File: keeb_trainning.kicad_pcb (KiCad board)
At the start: 2 copper layers, 0 parts

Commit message: :construction: WIP: Redraw wires
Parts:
- added D1: Diode, ScottoKeebs_Components:Diode_SOD-123, F.Cu at (72.5, 81.9)
- added D10: Diode, ScottoKeebs_Components:Diode_SOD-123, F.Cu at (59.1, 87.7)
- added D11: Diode, ScottoKeebs_Components:Diode_SOD-123, F.Cu at (72.5, 93.4)
- added D12: Diode, ScottoKeebs_Components:Diode_SOD-123, F.Cu at (69.2, 93.4)
- added D13: Diode, ScottoKeebs_Components:Diode_SOD-123, F.Cu at (65.8, 93.4)
- added D14: Diode, ScottoKeebs_Components:Diode_SOD-123, F.Cu at (62.5, 93.4)
- added D15: Diode, ScottoKeebs_Components:Diode_SOD-123, F.Cu at (59.1, 93.4)
- added D16: Diode, ScottoKeebs_Components:Diode_SOD-123, F.Cu at (72.5, 99.2)
- added D17: Diode, ScottoKeebs_Components:Diode_SOD-123, F.Cu at (69.2, 99.2)
- added D18: Diode, ScottoKeebs_Components:Diode_SOD-123, F.Cu at (65.8, 99.2)
- added D19: Diode, ScottoKeebs_Components:Diode_SOD-123, F.Cu at (62.5, 99.2)
- added D2: Diode, ScottoKeebs_Components:Diode_SOD-123, F.Cu at (69.2, 81.9)
- added D20: Diode, ScottoKeebs_Components:Diode_SOD-123, F.Cu at (59.1, 99.2)
- added D3: Diode, ScottoKeebs_Components:Diode_SOD-123, F.Cu at (65.8, 81.9)
- added D4: Diode, ScottoKeebs_Components:Diode_SOD-123, F.Cu at (62.5, 81.9)
- added D5: Diode, ScottoKeebs_Components:Diode_SOD-123, F.Cu at (59.1, 81.9)
- added D6: Diode, ScottoKeebs_Components:Diode_SOD-123, F.Cu at (72.5, 87.7)
- added D7: Diode, ScottoKeebs_Components:Diode_SOD-123, F.Cu at (69.2, 87.7)
- added D8: Diode, ScottoKeebs_Components:Diode_SOD-123, F.Cu at (65.8, 87.7)
- added D9: Diode, ScottoKeebs_Components:Diode_SOD-123, F.Cu at (62.5, 87.7)
- added S1: Keyswitch, ScottoKeebs_Choc:Choc_V2, F.Cu at (88.2, 53.7)
- added S10: Keyswitch, ScottoKeebs_Choc:Choc_V2, F.Cu at (145.7, 69.7)
- added S11: Keyswitch, ScottoKeebs_Choc:Choc_V2, F.Cu at (166.2, 74.2)
- added S12: Keyswitch, ScottoKeebs_Choc:Choc_V2, F.Cu at (185.2, 75.8)
- added S13: Keyswitch, ScottoKeebs_Choc:Choc_V2, F.Cu at (87.7, 89.7)
- added S14: Keyswitch, ScottoKeebs_Choc:Choc_V2, F.Cu at (106.7, 89.8)
- added S15: Keyswitch, ScottoKeebs_Choc:Choc_V2, F.Cu at (126.2, 83.8)
- added S16: Keyswitch, ScottoKeebs_Choc:Choc_V2, F.Cu at (145.7, 87.8)
- added S17: Keyswitch, ScottoKeebs_Choc:Choc_V2, F.Cu at (166.2, 92.3)
- added S18: Keyswitch, ScottoKeebs_Choc:Choc_V2, F.Cu at (185.2, 94.3)
- added S19: Keyswitch, ScottoKeebs_Choc:Choc_V2_1.50u_90deg, F.Cu at (82.7, 116.3)
- added S2: Keyswitch, ScottoKeebs_Choc:Choc_V2, F.Cu at (107.2, 53.7)
- added S20: Keyswitch, ScottoKeebs_Choc:Choc_V2_1.50u_90deg, F.Cu at (61.7, 118.8)
- added S3: Keyswitch, ScottoKeebs_Choc:Choc_V2, F.Cu at (126.2, 48.2)
- added S4: Keyswitch, ScottoKeebs_Choc:Choc_V2, F.Cu at (145.7, 52.2)
- added S5: Keyswitch, ScottoKeebs_Choc:Choc_V2, F.Cu at (166.2, 56.7)
- added S6: Keyswitch, ScottoKeebs_Choc:Choc_V2, F.Cu at (185.2, 57.7)
- added S7: Keyswitch, ScottoKeebs_Choc:Choc_V2, F.Cu at (88.2, 71.8)
- added S8: Keyswitch, ScottoKeebs_Choc:Choc_V2, F.Cu at (107.2, 71.8)
- added S9: Keyswitch, ScottoKeebs_Choc:Choc_V2, F.Cu at (126.2, 66.2)
- added U1: Universal_Pro_Micro, custom:Universal_Pro_Micro_Footprint, F.Cu at (65.6, 61.2)
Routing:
- net col5: track 0.00 -> 283.7 mm
- net col4: track 0.00 -> 280.5 mm, vias 0 -> 1
- net col2: track 0.00 -> 201.3 mm
- net col1: track 0.00 -> 178.6 mm
- net col3: track 0.00 -> 173.4 mm, vias 0 -> 1
- net col0: track 0.00 -> 152.5 mm
- net row2: track 0.00 -> 70.8 mm, vias 0 -> 2
- net row1: track 0.00 -> 69.3 mm, vias 0 -> 4
- net row0: track 0.00 -> 65.5 mm, vias 0 -> 2
- net row3: track 0.00 -> 55.1 mm
- added copper zone on B.Cu, net (none)
- added copper zone on F.Cu, net (none)
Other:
- board outline added: 159 x 108.5 mm

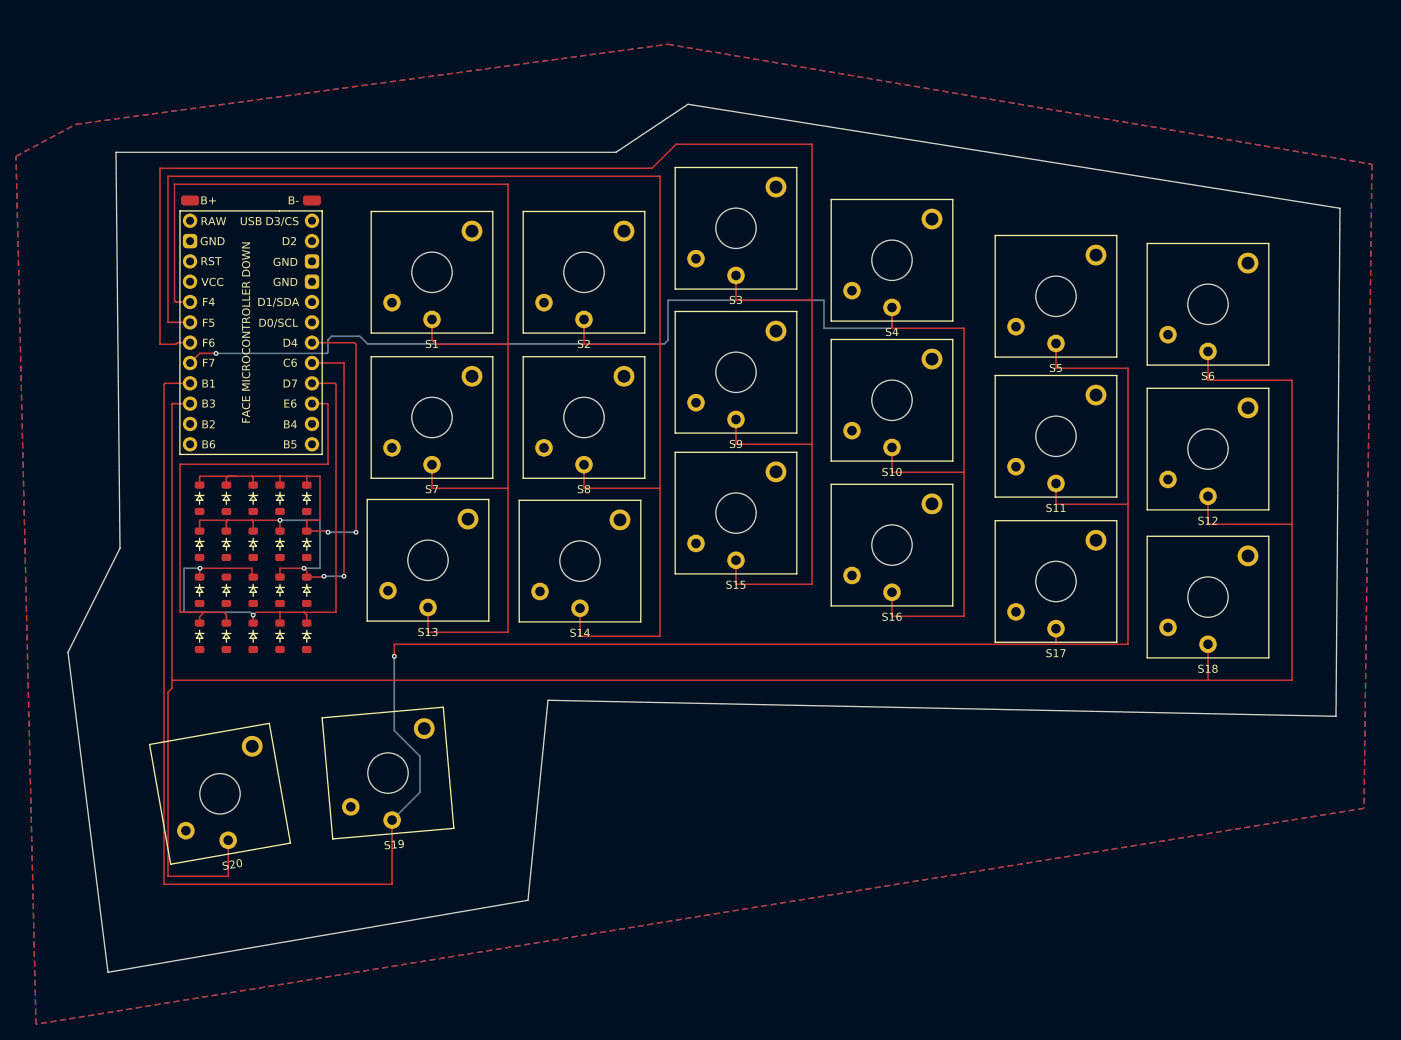
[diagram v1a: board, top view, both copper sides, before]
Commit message: :construction: WIP: Added hotswap
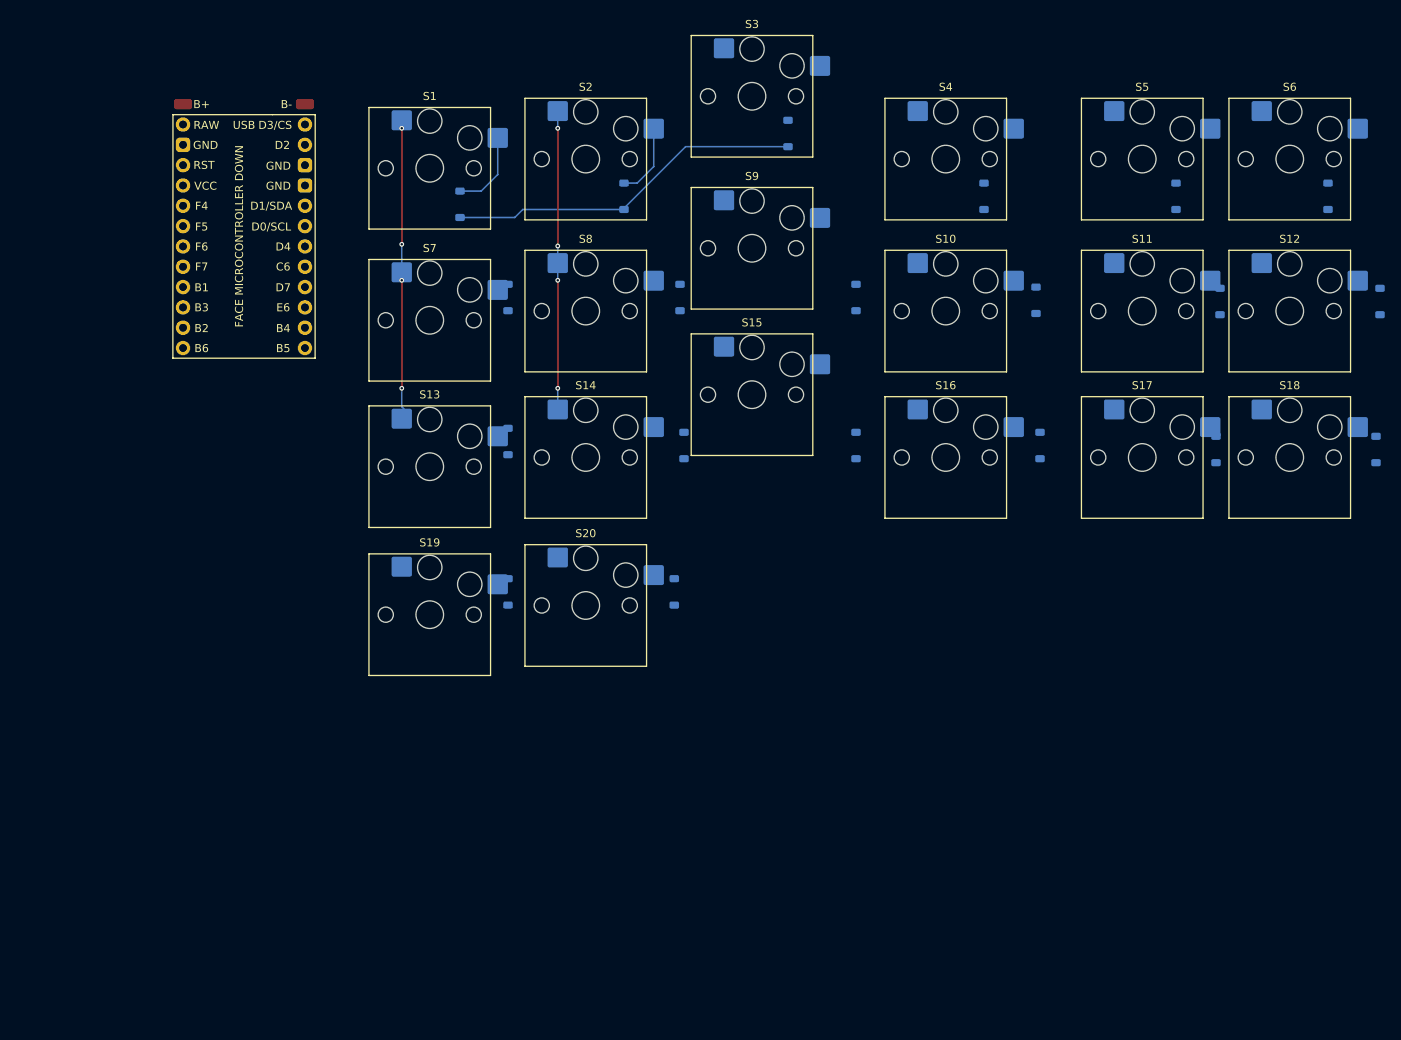
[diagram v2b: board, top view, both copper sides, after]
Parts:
- D1, D10, D11, D12, D13, D14, D15, D16, D17, D18, D19, D2, D20, D3, D4, D5, D6, D7, D8, D9: moved to B.Cu
- S1, S10, S11, S12, S13, S14, S15, S16, S17, S18, S2, S3, S4, S5, S6, S7, S8, S9: footprint ScottoKeebs_Choc:Choc_V2 -> ScottoKeebs_Hotswap:Hotswap_Choc_V1
- S19, S20: footprint ScottoKeebs_Choc:Choc_V2_1.50u_90deg -> ScottoKeebs_Hotswap:Hotswap_Choc_V1
- moved D18 142.3 mm to (206.2, 75.8)
- moved D12 142.2 mm to (206.7, 57.3)
- moved D6 134.9 mm to (200.2, 44.2), turned to 90 degrees
- moved D5 127.8 mm to (181.2, 44.2), turned to 90 degrees
- moved D11 119.7 mm to (186.7, 57.3)
- moved D17 119.3 mm to (186.2, 75.8)
- moved D10 108.9 mm to (163.7, 57.2), turned to 90 degrees
- moved D4 101.9 mm to (157.2, 44.2), turned to 90 degrees
- moved D16 94.7 mm to (164.2, 75.3)
- moved D9 84.5 mm to (141.2, 56.8), turned to 90 degrees
- moved D15 84.0 mm to (141.2, 75.3)
- moved D3 80.9 mm to (132.7, 36.3), turned to 90 degrees
- moved D8 61.6 mm to (119.2, 56.8), turned to 90 degrees
- moved D14 60.0 mm to (119.7, 75.3)
- moved D20 59.6 mm to (118.5, 93.6)
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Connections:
- U1 pad 10: row3 -> unconnected-(U1-P0.11-Pad10)
- U1 pad 17: col0 -> unconnected-(U1-P0.31-LF-Pad17)
- U1 pad 18: col1 -> unconnected-(U1-P0.29-LF-Pad18)
- U1 pad 19: col2 -> unconnected-(U1-P0.02-LF-Pad19)
- U1 pad 20: col3 -> unconnected-(U1-P1.15-LF-Pad20)
- U1 pad 21: col4 -> unconnected-(U1-P1.13-LF-Pad21)
- U1 pad 22: col5 -> unconnected-(U1-P1.11-LF-Pad22)
- U1 pad 7: row0 -> unconnected-(U1-P0.22-Pad7)
- U1 pad 8: row1 -> unconnected-(U1-P0.24-Pad8)
- U1 pad 9: row2 -> unconnected-(U1-P1.00-Pad9)
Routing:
- net col5: track 283.7 -> 0.00 mm
- net col4: track 280.5 -> 0.00 mm, vias 1 -> 0
- net col2: track 201.3 -> 0.00 mm
- net col3: track 173.4 -> 0.00 mm, vias 1 -> 0
- net col1: track 178.6 -> 37.8 mm, vias 0 -> 4
- net col0: track 152.5 -> 37.4 mm, vias 0 -> 4
- net row2: track 70.8 -> 0.00 mm, vias 2 -> 0
- net row1: track 69.3 -> 0.00 mm, vias 4 -> 0
- net row3: track 55.1 -> 0.00 mm
- net row0: track 65.5 -> 44.8 mm, vias 2 -> 0
- net Net-(D1-A): track 0.00 -> 10.2 mm
- net Net-(D2-A): track 0.00 -> 9.31 mm
- removed copper zone on B.Cu, net (none)
- removed copper zone on F.Cu, net (none)
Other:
- board outline removed
